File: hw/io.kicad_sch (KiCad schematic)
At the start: 12 parts, among them J1 Conn_02x08_Odd_Even, J3 Conn_02x08_Odd_Even, U11 74HC138, U5 74HC86, U6 74HC245, U7 74HC245, U8 74HC02, U9 74HC00

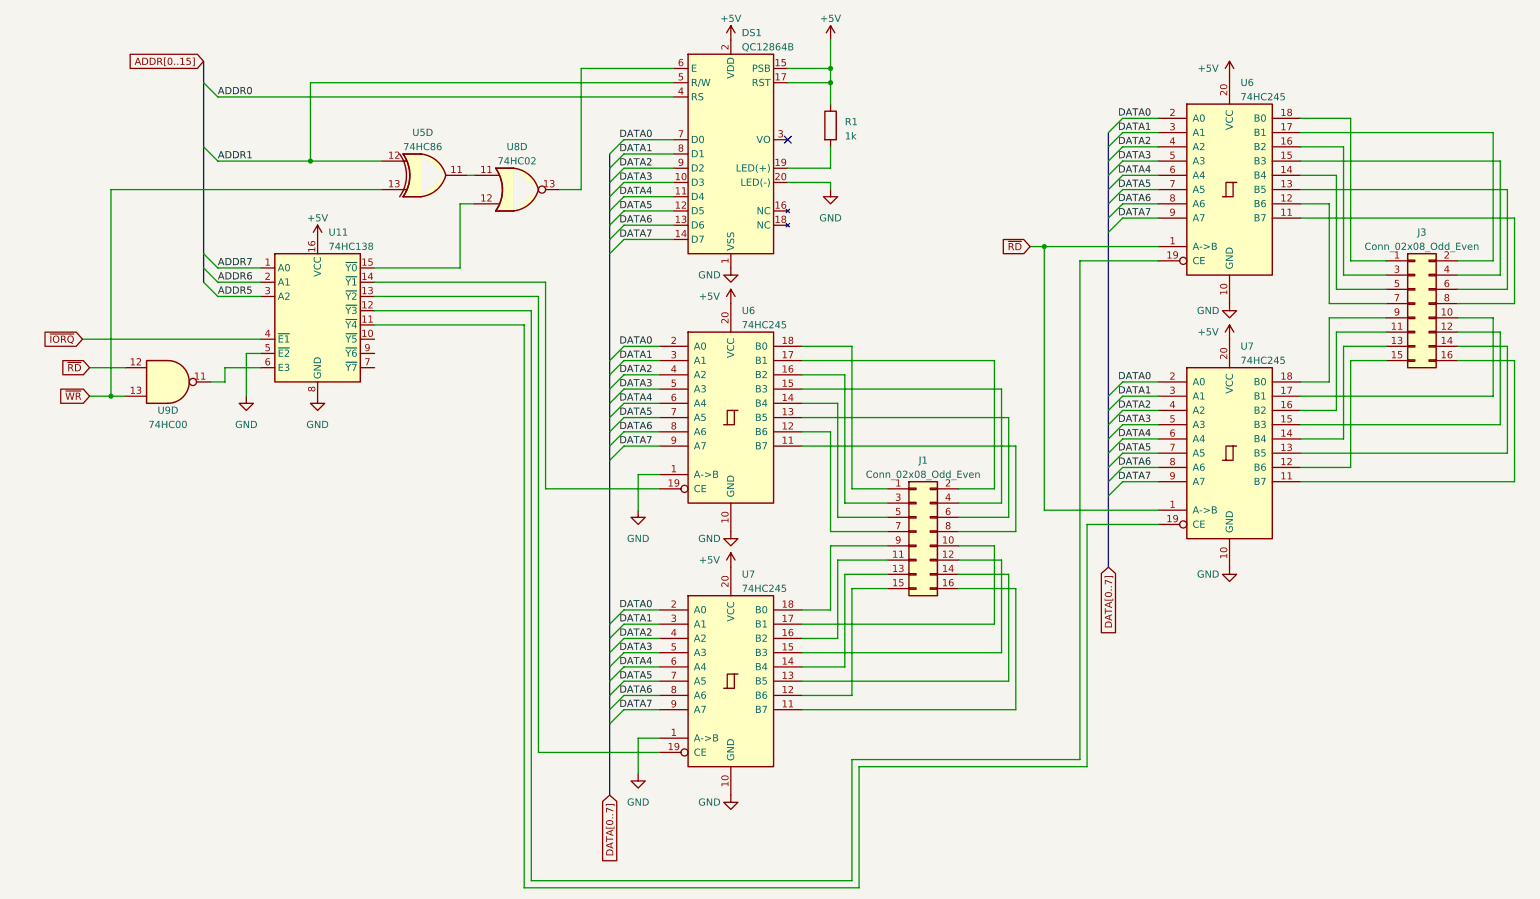
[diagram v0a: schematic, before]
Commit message: Work on scmenatic and PCB
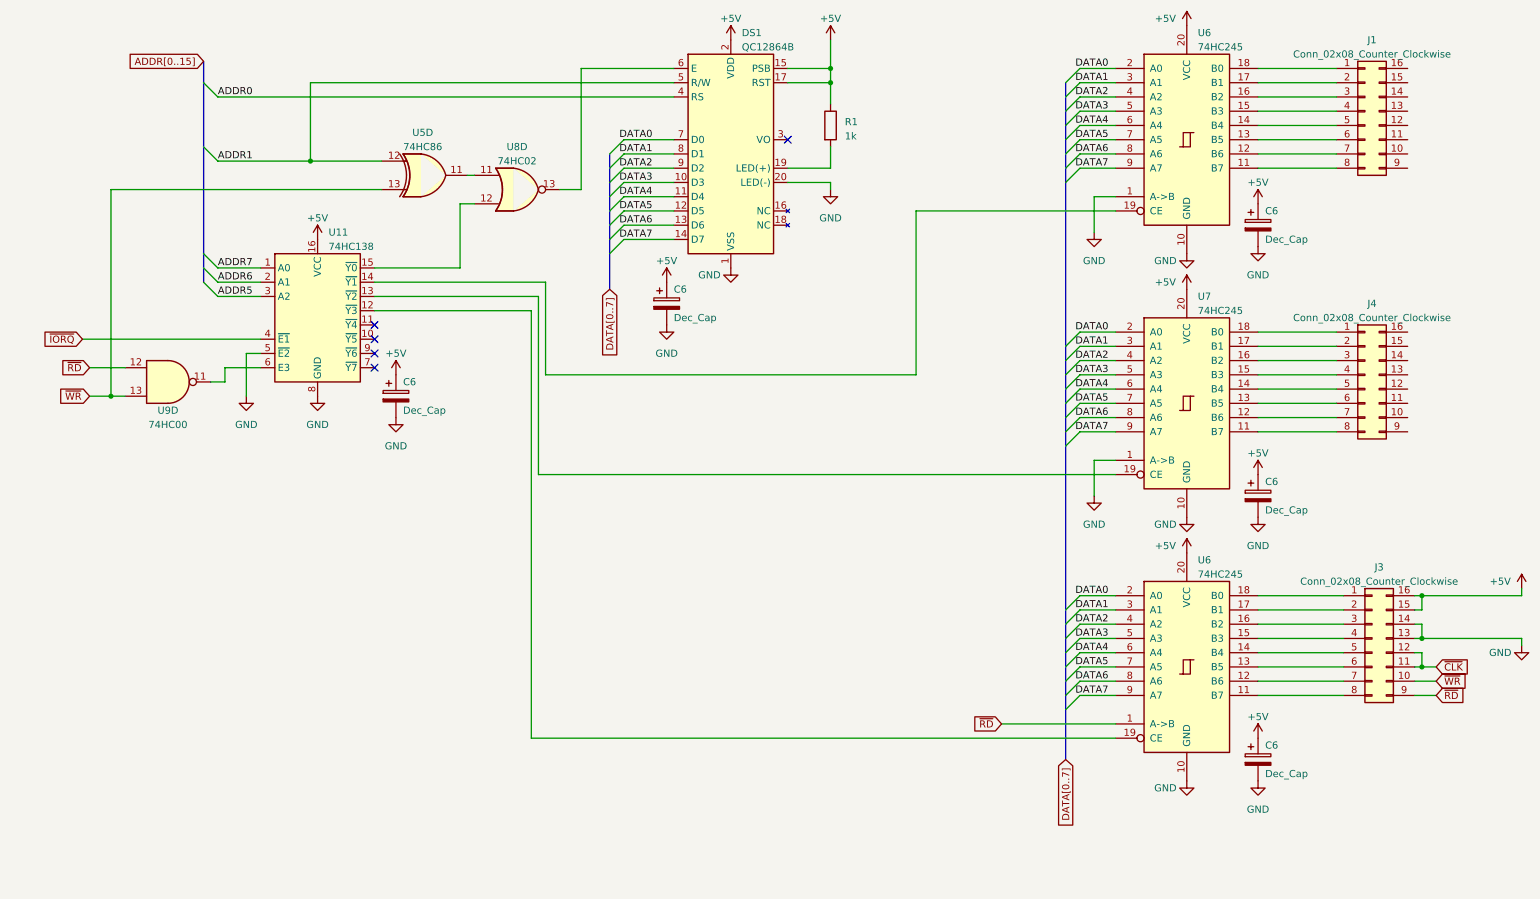
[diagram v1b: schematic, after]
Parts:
- removed J1, J3: Conn_02x08_Odd_Even, Connector_PinHeader_2.54mm:PinHeader_2x08_P2.54mm_Vertical, symbol Connector_Generic:Conn_02x08_Odd_Even
- removed U7 (x2): 74HC245, Package_DIP:DIP-20_W7.62mm_Socket_LongPads, symbol 74xx:74HC245
- added C6 (x5): Dec_Cap, Capacitor_THT:C_Disc_D3.0mm_W1.6mm_P2.50mm, symbol z80mgc:Dec_Cap
- added J1, J3, J4: Conn_02x08_Counter_Clockwise, z80mgc:PinHeader_2x08_P2.54mm_Vertical, symbol Connector_Generic:Conn_02x08_Counter_Clockwise
- added U7: 74HC245, Package_DIP:DIP-20_W7.62mm_Socket_LongPads, symbol 74xx:74HC245
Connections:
- net +5V: now also C6.1, C6.1, C6.1, C6.1, C6.1, J3.15 (Pin_15), J3.16 (Pin_16), U7.20 (VCC)
- net DATA0: now also U7.2 (A0)
- net DATA1: now also U7.3 (A1)
- net DATA2: now also U7.4 (A2)
- net DATA3: now also U7.5 (A3)
- net DATA4: now also U7.6 (A4)
- net DATA5: now also U7.7 (A5)
- net DATA6: now also U7.8 (A6)
- net DATA7: now also U7.9 (A7)
- net GND: now also C6.2, C6.2, C6.2, C6.2, C6.2, J3.13 (Pin_13), J3.14 (Pin_14), U7.1 (A->B), U7.10 (GND)
- net ~{RD}: now also J3.9 (Pin_9)
- net ~{WR}: now also J3.10 (Pin_10)
- net at U6.18 (B0): now also J1.1 (Pin_1)
- net at U6.17 (B1): now also J1.2 (Pin_2)
- net at U6.16 (B2): now also J1.3 (Pin_3)
- net at U6.15 (B3): now also J1.4 (Pin_4)
- net at U6.14 (B4): now also J1.5 (Pin_5)
- net at U6.13 (B5): now also J1.6 (Pin_6)
- net at U6.12 (B6): now also J1.7 (Pin_7)
- net at U6.11 (B7): now also J1.8 (Pin_8)
- net at U6.18 (B0): now also J3.1 (Pin_1)
- net at U6.17 (B1): now also J3.2 (Pin_2)
- net at U6.16 (B2): now also J3.3 (Pin_3)
- net at U6.15 (B3): now also J3.4 (Pin_4)
- net at U6.14 (B4): now also J3.5 (Pin_5)
- net at U6.13 (B5): now also J3.6 (Pin_6)
- net at U6.12 (B6): now also J3.7 (Pin_7)
- net at U6.11 (B7): now also J3.8 (Pin_8)
- net at U11.13 (~{Y2}): now also U7.19 (CE)
- new net: J4.1 (Pin_1), U7.18 (B0)
- new net: J4.2 (Pin_2), U7.17 (B1)
- new net: J4.3 (Pin_3), U7.16 (B2)
- new net: J4.4 (Pin_4), U7.15 (B3)
- new net: J4.5 (Pin_5), U7.14 (B4)
- new net: J4.6 (Pin_6), U7.13 (B5)
- new net: J4.7 (Pin_7), U7.12 (B6)
- new net: J4.8 (Pin_8), U7.11 (B7)
- new net ~{CLK}: J3.11 (Pin_11), J3.12 (Pin_12)
- no-connect marks 1 -> 5
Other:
- moved on the sheet: U6
